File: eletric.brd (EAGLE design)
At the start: 100 x 106.7 mm, 15 parts, among them U1 ATTINY85-20PU

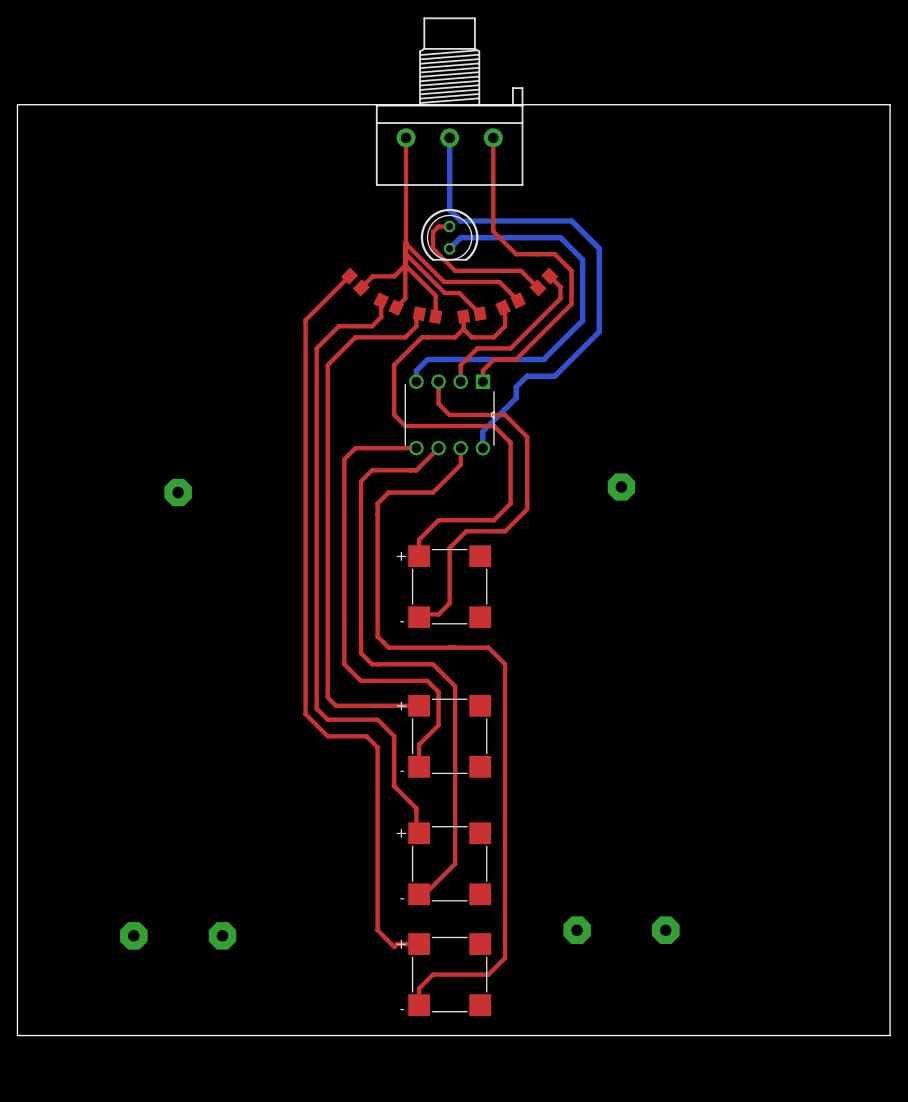
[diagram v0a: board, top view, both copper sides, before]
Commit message: pcb improve layout
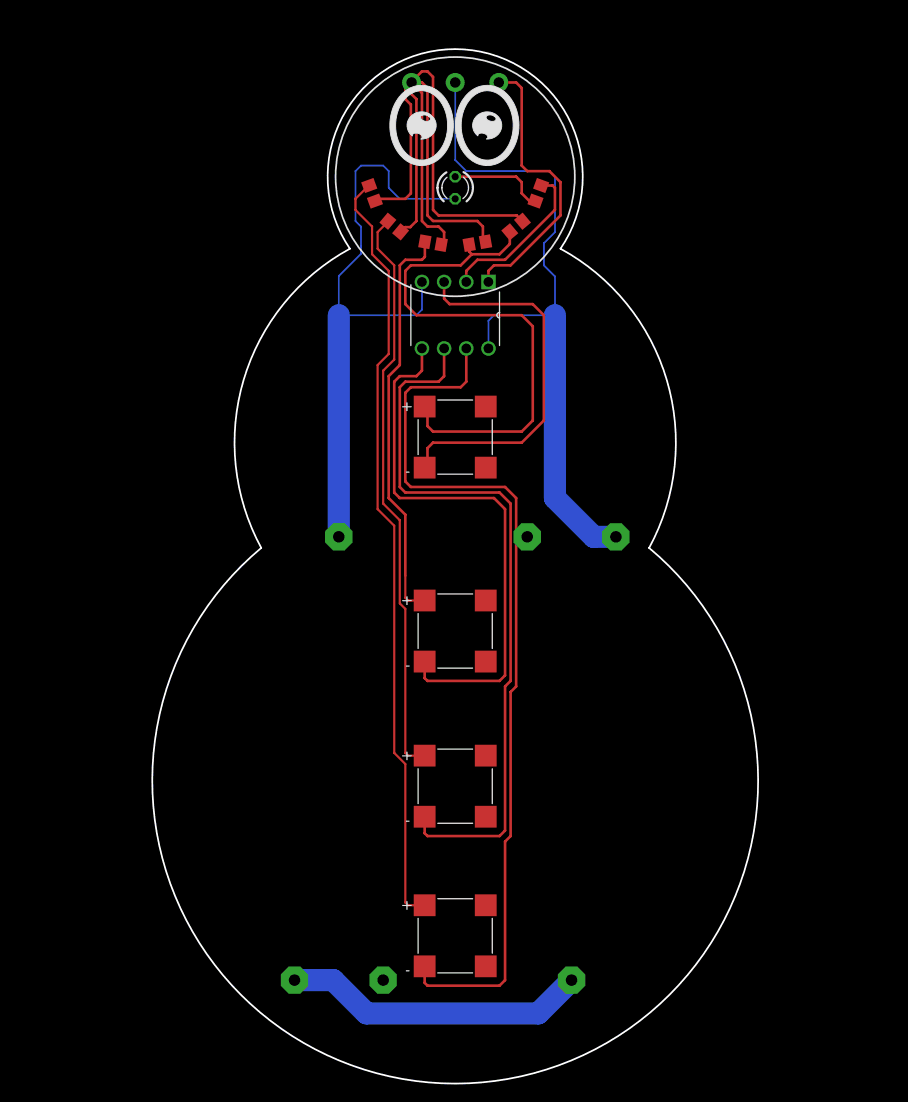
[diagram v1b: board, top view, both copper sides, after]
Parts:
- removed LED2: (no value), led:LED5MM
- added LED1: (no value), led:LED3MM
- moved G2 19.1 mm to (36.8, 31.8)
- moved LS1 17.2 mm to (50.2, 68.6)
- moved LS3 12.1 mm to (50.2, 46.4)
- moved U1 11.4 mm to (46.4, 78.7)
- moved R2 10.3 mm to (40.6, 96.5), turned to 110 degrees
- moved R7 10.2 mm to (59.7, 96.5), turned to 250 degrees
- moved LS4 8.91 mm to (50.2, 28.6)
- moved R3 8.91 mm to (43.2, 92.7), turned to 140 degrees
- moved R6 8.91 mm to (57.1, 92.7), turned to 220 degrees
- moved R4 8.28 mm to (47.6, 90.8)
- moved R5 8.28 mm to (52.7, 90.8)
- moved G1 8.08 mm to (63.5, 31.8), turned to 270 degrees
- moved R1 6.38 mm to (50.2, 109.2), flipped to the bottom
- moved LS2 4.49 mm to (50.2, 11.4)
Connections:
- net GND: now also LED1.K; no longer LED2.K
- net N$5: now also LED1.A; no longer LED2.A
- net RESET: now also R1.3; no longer R1.1
- net VOLUME: now also R1.1; no longer R1.3
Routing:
- net VOLUME: track 62.9 -> 112.0 mm
- net N$1: track 0.00 -> 34.9 mm
- net GND: track 46.5 -> 70.6 mm
- net VCC: track 57.5 -> 78.9 mm
- net N$4: track 62.5 -> 47.2 mm
- net BUZER_HARMONY_2: track 68.4 -> 82.9 mm
- net BUZER_HARMONY_1: track 91.9 -> 102.2 mm
- net BUZER_HARMONY_3: track 53.9 -> 63.0 mm
- net N$2: track 74.5 -> 66.1 mm
- net RESET: track 40.0 -> 33.0 mm
- net N$5: track 18.0 -> 11.1 mm
- net N$6: track 60.4 -> 62.7 mm
- net LED: track 19.6 -> 18.6 mm
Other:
- board size 100 x 106.7 mm -> 69.4 x 118.6 mm
